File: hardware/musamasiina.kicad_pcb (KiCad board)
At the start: 2 copper layers, 50 x 50 mm, 92 parts, among them P1 USB_OTG, P2 CONN_02X05, P3 CONN_02X03, P4 CONN_01X06, P5 CONN_01X03, P6 CONN_01X03, P7 CONN_01X03, U1 WT32, U2 MIC5233-3.3, U3 LTC6257, U4 TPS22860

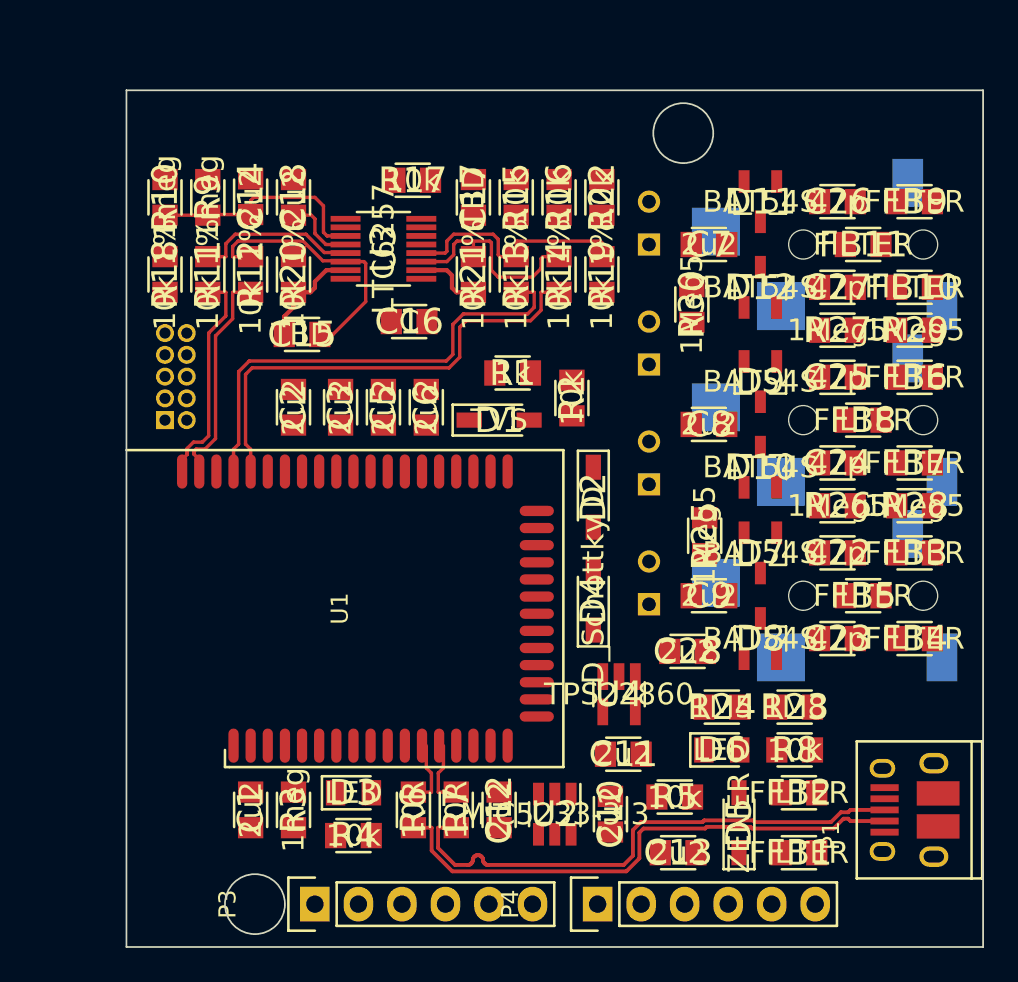
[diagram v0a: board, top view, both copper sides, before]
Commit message: Layout board
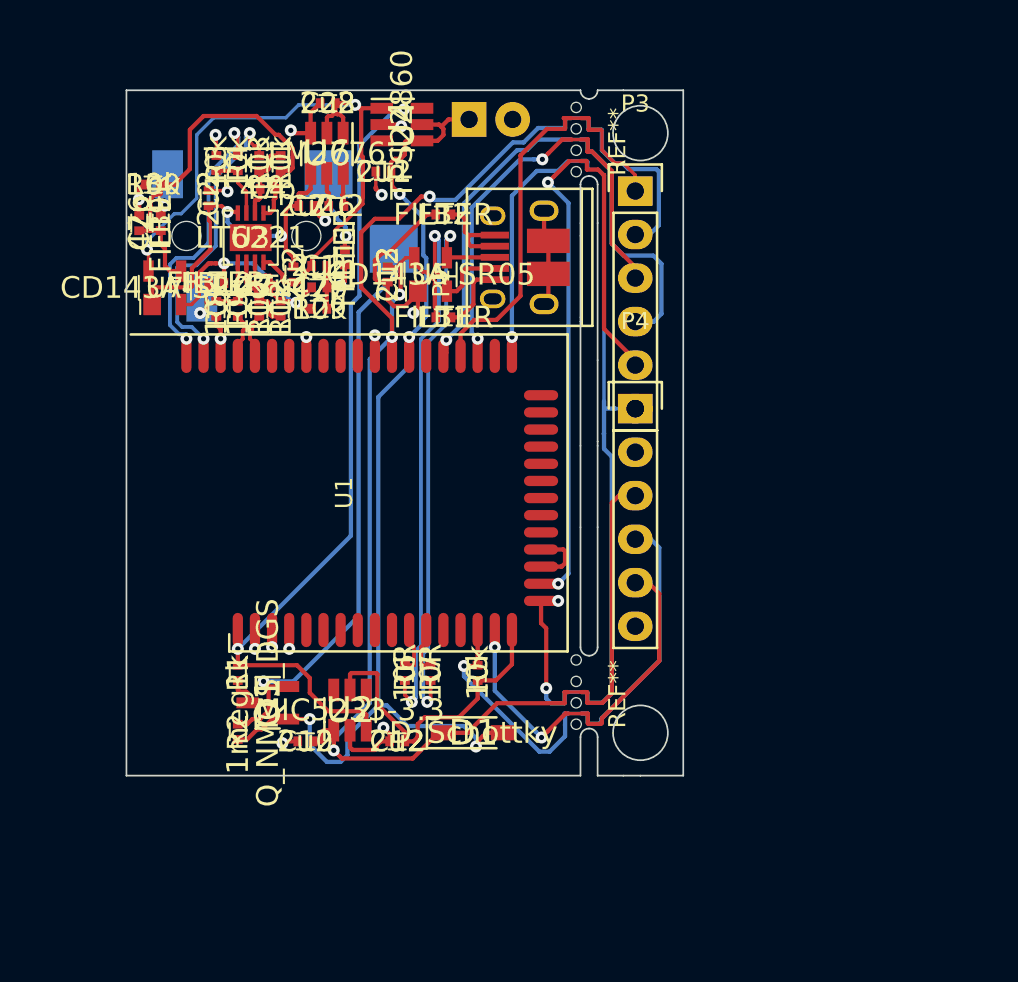
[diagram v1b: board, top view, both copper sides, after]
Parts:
- removed C14, C18, C8, C9: 2u2, footprints:SMD0805-CAP-M
- removed C15, C17: TBD, footprints:SMD0805-CAP-M
- removed C16: C, footprints:SMD0805-CAP-M
- removed C19, C20, C21: 470u, footprints:C_Radial_D6.3_L13_P2-5_Bent
- removed C22, C23, C24, C25: 47p, footprints:SMD0805-CAP-M
- removed D10, D11, D12, D7, D8, D9: BAT54S, footprints:SOT23-M
- removed D2: D, footprints:SOD323-M
- removed D3, D6: LED, footprints:SMD0805-LED-M
- removed D4: D_Schottky, footprints:SOD323-M
- removed D5: ZENER, footprints:SOD323-M
- removed FB3, FB4, FB5, FB6, FB7, FB8: FILTER, footprints:SMD0805-FERRITE-M
- removed P5, P6, P7: CONN_01X03, footprints:SMD_3-5mm_jack_CUI-SJ-352X-SMT
- removed R14, R18, R19, R20, R21: 10k 1%, footprints:SMD0805-RES-M
- removed R15, R16, R17, R22: 10k, footprints:SMD0805-RES-M
- removed R23: 1M8, footprints:SMD0805-RES-M
- removed R24: 1M5, footprints:SMD0805-RES-M
- removed R25, R26, R27, R28: 1Meg5, footprints:SMD0805-RES-M
- added BT1: Battery, Pin_Headers:Pin_Header_Angled_1x02, B.Cu at (130.0, 51.7)
- added Q1: Q_NMOS_DGS, footprints:SOT23-M, F.Cu at (118.2, 85.8)
- added REF**: BREAKAWAY_5, BREAKAWAY_5, F.Cu at (136.2, 53.0)
- added REF**: BREAKAWAY_5, BREAKAWAY_5, F.Cu at (136.2, 85.2)
- added U5: CD143A-SR05, footprints:SOT143-N, F.Cu at (127.8, 60.8)
- added U6: LM2776, footprints:SOT23-6-M, F.Cu at (121.7, 53.7)
- added U7: CD143A-SR05, footprints:SOT143-N, F.Cu at (112.2, 61.5)
- C1, C10, C11, C12, C13, C2, C26, C27, C28, C3, C6, C7: footprint footprints:SMD0805-CAP-M -> footprints:SMD0402-CAP-N
- C4: value AFK477M10F24T-F -> 47p; footprint footprints:C_Radial_D6.3_L13_P2-5_Bent -> footprints:SMD0402-CAP-N; moved to F.Cu
- C5: value 2u2 -> 47p; footprint footprints:SMD0805-CAP-M -> footprints:SMD0402-CAP-N
- D1: value TVS -> D_Schottky
- FB1, FB10, FB11, FB2, FB9: footprint footprints:SMD0805-FERRITE-M -> footprints:SMD0402-FERRITE-N
- P2: value CONN_02X05 -> CONN_01X04; footprint Pin_Headers:Pin_Header_Straight_2x05_Pitch1.27mm -> footprints:SMD_3-5mm_jack_CUI-SJ-352X-SMT
- R1, R4, R5, R6, R7, R8: footprint footprints:SMD0805-RES-M -> footprints:SMD0402-RES-N
- R10, R3, R9: value 1meg -> 10k; footprint footprints:SMD0805-RES-M -> footprints:SMD0402-RES-N
- R11, R12, R13: value 10k 1% -> 10k; footprint footprints:SMD0805-RES-M -> footprints:SMD0402-RES-N
- R2: value 10k -> 1meg; footprint footprints:SMD0805-RES-M -> footprints:SMD0402-RES-N
- R29, R30: value 1Meg5 -> 10k; footprint footprints:SMD0805-RES-M -> footprints:SMD0402-RES-N
- U3: value LTC6257 -> LT6221; footprint footprints:MSOP16-05mm-M -> footprints:DFN-8-EP-0_5mm_3x3mm-N
- U4: footprint footprints:SOT23-5-M -> footprints:SOT23-6-M
- moved P3 45.6 mm to (139.7, 55.9), turned to 0 degrees
- moved FB9 44.0 mm to (112.0, 57.7), turned to 90 degrees
- moved R8 42.5 mm to (115.2, 62.8), turned to 270 degrees
- moved C26 40.8 mm to (110.8, 57.8), turned to 90 degrees
- moved FB10 40.8 mm to (115.2, 61.2), turned to 180 degrees
- moved R4 39.8 mm to (116.5, 54.2), turned to 90 degrees
- moved FB2 39.6 mm to (128.5, 57.2)
- moved P1 39.5 mm to (133.0, 59.8)
- moved C28 38.3 mm to (121.8, 50.8), turned to 180 degrees
- moved R3 38.0 mm to (115.2, 54.2), turned to 90 degrees
- moved C13 37.8 mm to (125.2, 60.8), turned to 270 degrees
- moved FB1 37.5 mm to (128.5, 63.2)
- moved C11 36.8 mm to (125.0, 54.8)
- moved U4 35.6 mm to (126.1, 52.0), turned to 270 degrees
- moved R29 34.8 mm to (121.2, 62.8)
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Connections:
- C1 pad 1: Net-(C1-Pad1) -> VAA
- C1 pad 2: GNDD -> GNDA
- C2 pad 1: GNDA -> VEE
- C2 pad 2: Net-(C2-Pad2) -> GNDA
- C3 pad 1: GNDA -> VAA
- C3 pad 2: Net-(C3-Pad2) -> VEE
- C4 pad 1: +BATT -> /Stereo out/LEFT_DEVICE
- C4 pad 2: GNDD -> Net-(C4-Pad2)
- C5 pad 1: /Line in/LEFT_DEVICE -> /Stereo out/RIGHT_DEVICE
- C5 pad 2: /IN_LEFT -> Net-(C5-Pad2)
- C6 pad 1: /Line in/RIGHT_DEVICE -> Net-(C6-Pad1)
- C6 pad 2: /IN_RIGHT -> Net-(C6-Pad2)
- C7 pad 1: VAA -> VEE
- D1 pad 1: +BATT -> +5V
- D1 pad 2: Net-(D1-Pad2) -> +BATT
- P2 pad 1: VDD -> /Stereo out/LEFT_CABLE
- P2 pad 2: /PREV -> /Stereo out/GROUND_CABLE
- P2 pad 3: /VOL- -> /Stereo out/RIGHT_CABLE
- P2 pad 4: /NEXT -> /AUDIO_SWITCH
- P3 pad 2: VDD -> +5V
- P4 pad 3: VDD -> +5V
- R1 pad 1: Net-(C1-Pad1) -> /Power Supply/ENABLE
- R1 pad 2: Net-(D1-Pad2) -> Net-(Q1-Pad3)
- R10 pad 1: Net-(C14-Pad1) -> Net-(C5-Pad2)
- R10 pad 2: GNDA -> /RO_N
- R11 pad 1: /Analog/LEFT_OPAMP+ -> /Stereo out/LEFT_DEVICE
- R11 pad 2: /Analog/LO_P -> Net-(C4-Pad2)
- R12 pad 1: /Analog/LEFT_OPAMP- -> /Stereo out/RIGHT_DEVICE
- R12 pad 2: /Analog/LO_N -> Net-(C5-Pad2)
- R13 pad 1: /Analog/RIGHT_OPAMP+ -> Net-(C4-Pad2)
- R13 pad 2: /Analog/RO_P -> /LO_N
- R2 pad 1: Net-(D3-Pad2) -> +BATT
- R2 pad 2: /Power Supply/ENABLE -> /AUDIO_SWITCH
- R3 pad 1: Net-(D3-Pad2) -> Net-(R3-Pad1)
- R3 pad 2: GNDD -> GNDA
- R4 pad 1: Net-(D3-Pad1) -> Net-(R3-Pad1)
- R4 pad 2: GNDD -> /LO_P
- R8 pad 1: +5V -> Net-(R8-Pad1)
- R8 pad 2: Net-(D6-Pad2) -> GNDA
- R9 pad 1: VAA -> Net-(R8-Pad1)
- R9 pad 2: Net-(C14-Pad1) -> /RO_P
- U1 pad 1: Net-(C1-Pad1) -> /Power Supply/ENABLE
- U1 pad 36: /Power Supply/CHRG -> /CHRG
- U1 pad 38: VCC -> +5V
- U1 pad 42: Net-(C3-Pad2) -> Net-(U1-Pad42)
- U1 pad 45: Net-(C2-Pad2) -> Net-(U1-Pad45)
- U1 pad 46: /Analog/RO_N -> /RO_N
- U1 pad 47: /Analog/RO_P -> /RO_P
- U1 pad 49: /Analog/LO_N -> /LO_N
- U1 pad 50: /Analog/LO_P -> /LO_P
- U1 pad 7: Net-(D3-Pad2) -> Net-(U1-Pad7)
- U3 pad 1: VCOM -> /Stereo out/LEFT_DEVICE
- U3 pad 2: VCOM -> Net-(C4-Pad2)
- U3 pad 3: Net-(C14-Pad1) -> Net-(R3-Pad1)
- U3 pad 4: VAA -> VEE
- U3 pad 5: /Analog/LEFT_OPAMP+ -> Net-(R8-Pad1)
- U3 pad 6: /Analog/LEFT_OPAMP- -> Net-(C5-Pad2)
- U3 pad 7: /Analog/LEFT_SE -> /Stereo out/RIGHT_DEVICE
- U3 pad 8: (no net) -> VAA
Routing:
- net +5V: track 0.00 -> 106.5 mm, vias 0 -> 4
- net GNDD: track 0.00 -> 82.6 mm, vias 0 -> 10
- net +BATT: track 0.00 -> 64.1 mm, vias 0 -> 4
- net /Power Supply/ENABLE: track 0.00 -> 49.7 mm, vias 0 -> 2
- net /RESET: track 0.00 -> 41.4 mm, vias 0 -> 2
- net VAA: track 4.43 -> 40.8 mm, vias 0 -> 2
- net /AUDIO_SWITCH: track 0.00 -> 34.5 mm, vias 0 -> 1
- net /MOSI: track 0.00 -> 33.0 mm, vias 0 -> 1
- net /RXD: track 0.00 -> 28.8 mm, vias 0 -> 1
- net /Analog/RO_P: track 27.7 -> 0.00 mm
- net /Analog/RO_N: track 27.7 -> 0.00 mm
- net /SCLK: track 0.00 -> 26.7 mm, vias 0 -> 2
- net /MISO: track 0.00 -> 25.4 mm
- net /Stereo out/LEFT_DEVICE: track 0.00 -> 24.1 mm
- net /TXD: track 0.00 -> 22.7 mm, vias 0 -> 2
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- added copper zone on In1.Cu, net GNDA
- added copper zone on In1.Cu, net GNDD
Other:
- board size 50 x 50 mm -> 32.5 x 40 mm
- copper layers 2 -> 4
- net class Default: clearance 0.2 -> 0.17
- net class Opamp_differential: clearance 0.15 -> 0.17
- net class USB_DATA: clearance 0.15 -> 0.17
- rule trace_clearance: 0.2 -> 0.17
- rule trace_min: 0.2 -> 0.18
- board text added: "BATTERY"
- board text added: "otso@ojousima.net"
- board text added: "poppimASiina TINY"
